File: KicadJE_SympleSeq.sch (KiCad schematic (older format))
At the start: 32 parts, among them J101 CV-Out, J102 Reset + Step, J103 CV-G8_Mod1, J104 CV-G8_Mod2, J105 Clk_Hold, J106 G8-Out, J107 Reset + Step 1-4, J108 Reset + Step 5-8, J109 CV-G8_Base, U101 TL082

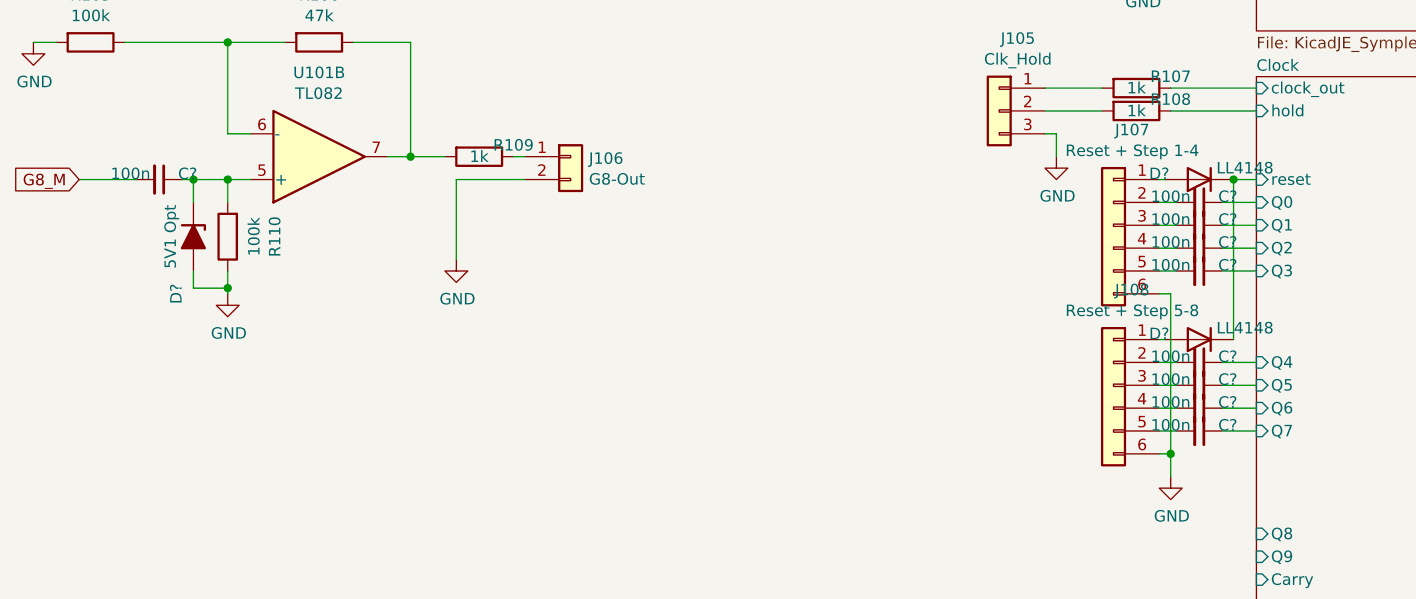
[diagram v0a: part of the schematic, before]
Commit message: ERC Rev B
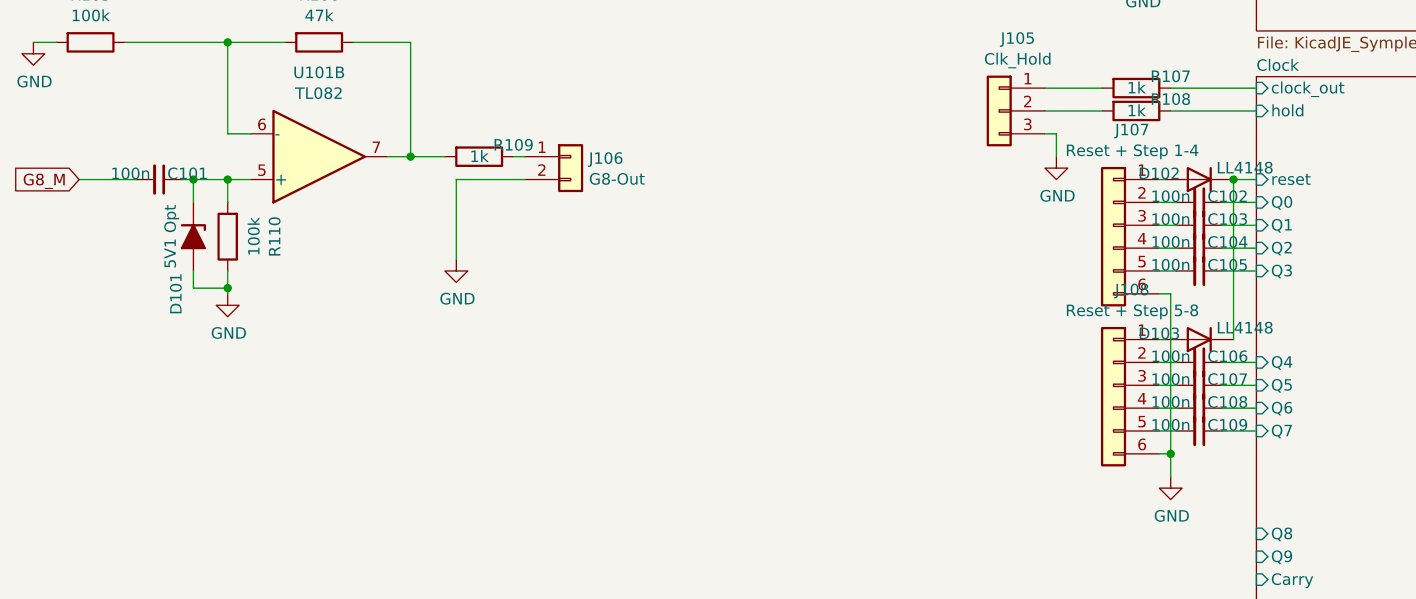
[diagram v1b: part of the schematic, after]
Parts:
- gave numbers to parts that had none: 12
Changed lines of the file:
@@
 	6575 3600 6600 3600
 $Comp
-L Device:C_Small C?
+L Device:C_Small C102
 U 1 1 5EA9D3AA
 P 6750 3700
-F 0 "C?" V 6725 3825 50  0000 C CNN
+F 0 "C102" V 6725 3825 50  0000 C CNN
 F 1 "100n" V 6725 3575 50  0000 C CNN
 F 2 "Capacitor_SMD:C_0805_2012Metric" H 6750 3700 50  0001 C CNN
@@
 	6575 3800 6650 3800
 $Comp
-L Device:C_Small C?
+L Device:C_Small C103
 U 1 1 5EA9ECF0
 P 6750 3800
-F 0 "C?" V 6725 3925 50  0000 C CNN
+F 0 "C103" V 6725 3925 50  0000 C CNN
 F 1 "100n" V 6725 3675 50  0000 C CNN
 F 2 "Capacitor_SMD:C_0805_2012Metric" H 6750 3800 50  0001 C CNN
@@
 	6850 3800 7000 3800
 $Comp
-L Device:C_Small C?
+L Device:C_Small C104
 U 1 1 5EA9F088
 P 6750 3900
-F 0 "C?" V 6725 4025 50  0000 C CNN
+F 0 "C104" V 6725 4025 50  0000 C CNN
 F 1 "100n" V 6725 3775 50  0000 C CNN
 F 2 "Capacitor_SMD:C_0805_2012Metric" H 6750 3900 50  0001 C CNN
@@
 	6850 3900 7000 3900
 $Comp
-L Device:C_Small C?
+L Device:C_Small C105
 U 1 1 5EA9F2B1
 P 6750 4000
-F 0 "C?" V 6725 4125 50  0000 C CNN
+F 0 "C105" V 6725 4125 50  0000 C CNN
 F 1 "100n" V 6725 3875 50  0000 C CNN
 F 2 "Capacitor_SMD:C_0805_2012Metric" H 6750 4000 50  0001 C CNN
@@
 	6850 4000 7000 4000
 $Comp
-L Device:C_Small C?
+L Device:C_Small C106
 U 1 1 5EA9F4B3
 P 6750 4400
-F 0 "C?" V 6725 4525 50  0000 C CNN
+F 0 "C106" V 6725 4525 50  0000 C CNN
 F 1 "100n" V 6725 4275 50  0000 C CNN
 F 2 "Capacitor_SMD:C_0805_2012Metric" H 6750 4400 50  0001 C CNN
@@
 	6850 4400 7000 4400
 $Comp
-L Device:C_Small C?
+L Device:C_Small C107
 U 1 1 5EA9F9A4
 P 6750 4500
-F 0 "C?" V 6725 4625 50  0000 C CNN
+F 0 "C107" V 6725 4625 50  0000 C CNN
 F 1 "100n" V 6725 4375 50  0000 C CNN
 F 2 "Capacitor_SMD:C_0805_2012Metric" H 6750 4500 50  0001 C CNN
@@
 	6850 4500 7000 4500
 $Comp
-L Device:C_Small C?
+L Device:C_Small C108
 U 1 1 5EA9FCDB
 P 6750 4600
-F 0 "C?" V 6725 4725 50  0000 C CNN
+F 0 "C108" V 6725 4725 50  0000 C CNN
 F 1 "100n" V 6725 4475 50  0000 C CNN
 F 2 "Capacitor_SMD:C_0805_2012Metric" H 6750 4600 50  0001 C CNN
@@
 	6850 4600 7000 4600
 $Comp
-L Device:C_Small C?
+L Device:C_Small C109
 U 1 1 5EA9FEC4
 P 6750 4700
-F 0 "C?" V 6725 4825 50  0000 C CNN
+F 0 "C109" V 6725 4825 50  0000 C CNN
 F 1 "100n" V 6725 4575 50  0000 C CNN
 F 2 "Capacitor_SMD:C_0805_2012Metric" H 6750 4700 50  0001 C CNN
@@
 	6850 4700 7000 4700
 $Comp
-L Device:C_Small C?
+L Device:C_Small C101
 U 1 1 5EAA1054
 P 2200 3600
-F 0 "C?" V 2175 3725 50  0000 C CNN
+F 0 "C101" V 2175 3725 50  0000 C CNN
 F 1 "100n" V 2175 3475 50  0000 C CNN
 F 2 "Capacitor_SMD:C_0805_2012Metric" H 2200 3600 50  0001 C CNN
@@
 P 6750 4300
 AR Path="/5C8BFBBC/5EBDB059" Ref="D?"  Part="1"
-AR Path="/5EBDB059" Ref="D?"  Part="1"
-F 0 "D?" H 6925 4275 50  0000 C CNN
+AR Path="/5EBDB059" Ref="D103"  Part="1"
+F 0 "D103" H 6925 4275 50  0000 C CNN
 F 1 "LL4148" H 6550 4250 50  0000 C CNN
 F 2 "Diode_SMD:D_MiniMELF" H 6750 4125 50  0001 C CNN
@@
 P 6750 3600
 AR Path="/5C8BFBBC/5EBDDE8B" Ref="D?"  Part="1"
-AR Path="/5EBDDE8B" Ref="D?"  Part="1"
-F 0 "D?" H 6925 3575 50  0000 C CNN
+AR Path="/5EBDDE8B" Ref="D102"  Part="1"
+F 0 "D102" H 6925 3575 50  0000 C CNN
 F 1 "LL4148" H 6550 3550 50  0000 C CNN
 F 2 "Diode_SMD:D_MiniMELF" H 6750 3425 50  0001 C CNN
@@
 P 2350 3850
 AR Path="/5C8BFBBC/5EBE23F1" Ref="D?"  Part="1"
-AR Path="/5EBE23F1" Ref="D?"  Part="1"
-F 0 "D?" H 2600 3775 50  0000 C CNN
+AR Path="/5EBE23F1" Ref="D101"  Part="1"
+F 0 "D101" H 2600 3775 50  0000 C CNN
 F 1 "5V1 Opt" H 2350 3750 50  0000 C CNN
 F 2 "Diode_SMD:D_MiniMELF" H 2350 3675 50  0001 C CNN

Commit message: AJ Footprints
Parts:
- C101, C102, C103, C104, C105, C106, C107, C108, C109: footprint Capacitor_SMD:C_0805_2012Metric -> AJ:C_0805_2012Metric_Pad1.15x1.40mm_HandSolder
- R101, R102, R103, R104, R105, R106, R107, R108, R109, R110: footprint Resistor_SMD:R_0805_2012Metric_Pad1.15x1.40mm_HandSolder -> AJ:R_0805_2012Metric_Pad1.15x1.40mm_HandSolder
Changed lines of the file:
@@
 F 0 "R106" V 2693 3000 50  0000 C CNN
 F 1 "47k" V 2784 3000 50  0000 C CNN
-F 2 "Resistor_SMD:R_0805_2012Metric_Pad1.15x1.40mm_HandSolder" V 2830 3000 50  0001 C CNN
+F 2 "AJ:R_0805_2012Metric_Pad1.15x1.40mm_HandSolder" V 2830 3000 50  0001 C CNN
 F 3 "~" H 2900 3000 50  0001 C CNN
 	1    2900 3000
@@
 F 0 "R105" V 1693 3000 50  0000 C CNN
 F 1 "100k" V 1784 3000 50  0000 C CNN
-F 2 "Resistor_SMD:R_0805_2012Metric_Pad1.15x1.40mm_HandSolder" V 1830 3000 50  0001 C CNN
+F 2 "AJ:R_0805_2012Metric_Pad1.15x1.40mm_HandSolder" V 1830 3000 50  0001 C CNN
 F 3 "~" H 1900 3000 50  0001 C CNN
 	1    1900 3000
@@
 F 0 "R110" V 2293 3850 50  0000 C CNN
 F 1 "100k" V 2384 3850 50  0000 C CNN
-F 2 "Resistor_SMD:R_0805_2012Metric_Pad1.15x1.40mm_HandSolder" V 2430 3850 50  0001 C CNN
+F 2 "AJ:R_0805_2012Metric_Pad1.15x1.40mm_HandSolder" V 2430 3850 50  0001 C CNN
 F 3 "~" H 2500 3850 50  0001 C CNN
 	1    2500 3850
@@
 F 0 "R107" V 6425 3350 50  0000 C CNN
 F 1 "1k" V 6475 3200 50  0000 C CNN
-F 2 "Resistor_SMD:R_0805_2012Metric_Pad1.15x1.40mm_HandSolder" V 6405 3200 50  0001 C CNN
+F 2 "AJ:R_0805_2012Metric_Pad1.15x1.40mm_HandSolder" V 6405 3200 50  0001 C CNN
 F 3 "~" H 6475 3200 50  0001 C CNN
 	1    6475 3200
@@
 F 0 "R108" V 6425 3450 50  0000 C CNN
 F 1 "1k" V 6475 3300 50  0000 C CNN
-F 2 "Resistor_SMD:R_0805_2012Metric_Pad1.15x1.40mm_HandSolder" V 6405 3300 50  0001 C CNN
+F 2 "AJ:R_0805_2012Metric_Pad1.15x1.40mm_HandSolder" V 6405 3300 50  0001 C CNN
 F 3 "~" H 6475 3300 50  0001 C CNN
 	1    6475 3300
@@
 F 0 "R102" V 2693 1150 50  0000 C CNN
 F 1 "47k" V 2784 1150 50  0000 C CNN
-F 2 "Resistor_SMD:R_0805_2012Metric_Pad1.15x1.40mm_HandSolder" V 2830 1150 50  0001 C CNN
+F 2 "AJ:R_0805_2012Metric_Pad1.15x1.40mm_HandSolder" V 2830 1150 50  0001 C CNN
 F 3 "~" H 2900 1150 50  0001 C CNN
 	1    2900 1150
@@
 F 0 "R104" V 2293 2000 50  0000 C CNN
 F 1 "100k" V 2384 2000 50  0000 C CNN
-F 2 "Resistor_SMD:R_0805_2012Metric_Pad1.15x1.40mm_HandSolder" V 2430 2000 50  0001 C CNN
+F 2 "AJ:R_0805_2012Metric_Pad1.15x1.40mm_HandSolder" V 2430 2000 50  0001 C CNN
 F 3 "~" H 2500 2000 50  0001 C CNN
 	1    2500 2000
@@
 F 0 "R101" V 1693 1150 50  0000 C CNN
 F 1 "100k" V 1784 1150 50  0000 C CNN
-F 2 "Resistor_SMD:R_0805_2012Metric_Pad1.15x1.40mm_HandSolder" V 1830 1150 50  0001 C CNN
+F 2 "AJ:R_0805_2012Metric_Pad1.15x1.40mm_HandSolder" V 1830 1150 50  0001 C CNN
 F 3 "~" H 1900 1150 50  0001 C CNN
 	1    1900 1150
@@
 F 0 "R109" V 3550 3650 50  0000 C CNN
 F 1 "1k" V 3600 3500 50  0000 C CNN
-F 2 "Resistor_SMD:R_0805_2012Metric_Pad1.15x1.40mm_HandSolder" V 3530 3500 50  0001 C CNN
+F 2 "AJ:R_0805_2012Metric_Pad1.15x1.40mm_HandSolder" V 3530 3500 50  0001 C CNN
 F 3 "~" H 3600 3500 50  0001 C CNN
 	1    3600 3500
@@
 F 0 "R103" V 3550 1800 50  0000 C CNN
 F 1 "1k" V 3600 1650 50  0000 C CNN
-F 2 "Resistor_SMD:R_0805_2012Metric_Pad1.15x1.40mm_HandSolder" V 3530 1650 50  0001 C CNN
+F 2 "AJ:R_0805_2012Metric_Pad1.15x1.40mm_HandSolder" V 3530 1650 50  0001 C CNN
 F 3 "~" H 3600 1650 50  0001 C CNN
 	1    3600 1650
@@
 F 0 "C102" V 6725 3825 50  0000 C CNN
 F 1 "100n" V 6725 3575 50  0000 C CNN
-F 2 "Capacitor_SMD:C_0805_2012Metric" H 6750 3700 50  0001 C CNN
+F 2 "AJ:C_0805_2012Metric_Pad1.15x1.40mm_HandSolder" H 6750 3700 50  0001 C CNN
 F 3 "~" H 6750 3700 50  0001 C CNN
 	1    6750 3700
@@
 F 0 "C103" V 6725 3925 50  0000 C CNN
 F 1 "100n" V 6725 3675 50  0000 C CNN
-F 2 "Capacitor_SMD:C_0805_2012Metric" H 6750 3800 50  0001 C CNN
+F 2 "AJ:C_0805_2012Metric_Pad1.15x1.40mm_HandSolder" H 6750 3800 50  0001 C CNN
 F 3 "~" H 6750 3800 50  0001 C CNN
 	1    6750 3800
@@
 F 0 "C104" V 6725 4025 50  0000 C CNN
 F 1 "100n" V 6725 3775 50  0000 C CNN
-F 2 "Capacitor_SMD:C_0805_2012Metric" H 6750 3900 50  0001 C CNN
+F 2 "AJ:C_0805_2012Metric_Pad1.15x1.40mm_HandSolder" H 6750 3900 50  0001 C CNN
 F 3 "~" H 6750 3900 50  0001 C CNN
 	1    6750 3900
@@
 F 0 "C105" V 6725 4125 50  0000 C CNN
 F 1 "100n" V 6725 3875 50  0000 C CNN
-F 2 "Capacitor_SMD:C_0805_2012Metric" H 6750 4000 50  0001 C CNN
+F 2 "AJ:C_0805_2012Metric_Pad1.15x1.40mm_HandSolder" H 6750 4000 50  0001 C CNN
 F 3 "~" H 6750 4000 50  0001 C CNN
 	1    6750 4000
@@
 F 0 "C106" V 6725 4525 50  0000 C CNN
 F 1 "100n" V 6725 4275 50  0000 C CNN
-F 2 "Capacitor_SMD:C_0805_2012Metric" H 6750 4400 50  0001 C CNN
+F 2 "AJ:C_0805_2012Metric_Pad1.15x1.40mm_HandSolder" H 6750 4400 50  0001 C CNN
 F 3 "~" H 6750 4400 50  0001 C CNN
 	1    6750 4400
@@
 F 0 "C107" V 6725 4625 50  0000 C CNN
 F 1 "100n" V 6725 4375 50  0000 C CNN
-F 2 "Capacitor_SMD:C_0805_2012Metric" H 6750 4500 50  0001 C CNN
+F 2 "AJ:C_0805_2012Metric_Pad1.15x1.40mm_HandSolder" H 6750 4500 50  0001 C CNN
 F 3 "~" H 6750 4500 50  0001 C CNN
 	1    6750 4500
@@
 F 0 "C108" V 6725 4725 50  0000 C CNN
 F 1 "100n" V 6725 4475 50  0000 C CNN
-F 2 "Capacitor_SMD:C_0805_2012Metric" H 6750 4600 50  0001 C CNN
+F 2 "AJ:C_0805_2012Metric_Pad1.15x1.40mm_HandSolder" H 6750 4600 50  0001 C CNN
 F 3 "~" H 6750 4600 50  0001 C CNN
 	1    6750 4600
@@
 F 0 "C109" V 6725 4825 50  0000 C CNN
 F 1 "100n" V 6725 4575 50  0000 C CNN
-F 2 "Capacitor_SMD:C_0805_2012Metric" H 6750 4700 50  0001 C CNN
+F 2 "AJ:C_0805_2012Metric_Pad1.15x1.40mm_HandSolder" H 6750 4700 50  0001 C CNN
 F 3 "~" H 6750 4700 50  0001 C CNN
 	1    6750 4700
@@
 F 0 "C101" V 2175 3725 50  0000 C CNN
 F 1 "100n" V 2175 3475 50  0000 C CNN
-F 2 "Capacitor_SMD:C_0805_2012Metric" H 2200 3600 50  0001 C CNN
+F 2 "AJ:C_0805_2012Metric_Pad1.15x1.40mm_HandSolder" H 2200 3600 50  0001 C CNN
 F 3 "~" H 2200 3600 50  0001 C CNN
 	1    2200 3600

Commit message: AJ footprints updated
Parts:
- C101, C102, C103, C104, C105, C106, C107, C108, C109: footprint AJ:C_0805_2012Metric_Pad1.15x1.40mm_HandSolder -> AJ:C_0805_AJ
- R101, R102, R103, R104, R105, R106, R107, R108, R109, R110: footprint AJ:R_0805_2012Metric_Pad1.15x1.40mm_HandSolder -> AJ:R_0805_AJ
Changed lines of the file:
@@
 F 0 "R106" V 2693 3000 50  0000 C CNN
 F 1 "47k" V 2784 3000 50  0000 C CNN
-F 2 "AJ:R_0805_2012Metric_Pad1.15x1.40mm_HandSolder" V 2830 3000 50  0001 C CNN
+F 2 "AJ:R_0805_AJ" V 2830 3000 50  0001 C CNN
 F 3 "~" H 2900 3000 50  0001 C CNN
 	1    2900 3000
@@
 F 0 "R105" V 1693 3000 50  0000 C CNN
 F 1 "100k" V 1784 3000 50  0000 C CNN
-F 2 "AJ:R_0805_2012Metric_Pad1.15x1.40mm_HandSolder" V 1830 3000 50  0001 C CNN
+F 2 "AJ:R_0805_AJ" V 1830 3000 50  0001 C CNN
 F 3 "~" H 1900 3000 50  0001 C CNN
 	1    1900 3000
@@
 F 0 "R110" V 2293 3850 50  0000 C CNN
 F 1 "100k" V 2384 3850 50  0000 C CNN
-F 2 "AJ:R_0805_2012Metric_Pad1.15x1.40mm_HandSolder" V 2430 3850 50  0001 C CNN
+F 2 "AJ:R_0805_AJ" V 2430 3850 50  0001 C CNN
 F 3 "~" H 2500 3850 50  0001 C CNN
 	1    2500 3850
@@
 F 0 "R107" V 6425 3350 50  0000 C CNN
 F 1 "1k" V 6475 3200 50  0000 C CNN
-F 2 "AJ:R_0805_2012Metric_Pad1.15x1.40mm_HandSolder" V 6405 3200 50  0001 C CNN
+F 2 "AJ:R_0805_AJ" V 6405 3200 50  0001 C CNN
 F 3 "~" H 6475 3200 50  0001 C CNN
 	1    6475 3200
@@
 F 0 "R108" V 6425 3450 50  0000 C CNN
 F 1 "1k" V 6475 3300 50  0000 C CNN
-F 2 "AJ:R_0805_2012Metric_Pad1.15x1.40mm_HandSolder" V 6405 3300 50  0001 C CNN
+F 2 "AJ:R_0805_AJ" V 6405 3300 50  0001 C CNN
 F 3 "~" H 6475 3300 50  0001 C CNN
 	1    6475 3300
@@
 F 0 "R102" V 2693 1150 50  0000 C CNN
 F 1 "47k" V 2784 1150 50  0000 C CNN
-F 2 "AJ:R_0805_2012Metric_Pad1.15x1.40mm_HandSolder" V 2830 1150 50  0001 C CNN
+F 2 "AJ:R_0805_AJ" V 2830 1150 50  0001 C CNN
 F 3 "~" H 2900 1150 50  0001 C CNN
 	1    2900 1150
@@
 F 0 "R104" V 2293 2000 50  0000 C CNN
 F 1 "100k" V 2384 2000 50  0000 C CNN
-F 2 "AJ:R_0805_2012Metric_Pad1.15x1.40mm_HandSolder" V 2430 2000 50  0001 C CNN
+F 2 "AJ:R_0805_AJ" V 2430 2000 50  0001 C CNN
 F 3 "~" H 2500 2000 50  0001 C CNN
 	1    2500 2000
@@
 F 0 "R101" V 1693 1150 50  0000 C CNN
 F 1 "100k" V 1784 1150 50  0000 C CNN
-F 2 "AJ:R_0805_2012Metric_Pad1.15x1.40mm_HandSolder" V 1830 1150 50  0001 C CNN
+F 2 "AJ:R_0805_AJ" V 1830 1150 50  0001 C CNN
 F 3 "~" H 1900 1150 50  0001 C CNN
 	1    1900 1150
@@
 F 0 "R109" V 3550 3650 50  0000 C CNN
 F 1 "1k" V 3600 3500 50  0000 C CNN
-F 2 "AJ:R_0805_2012Metric_Pad1.15x1.40mm_HandSolder" V 3530 3500 50  0001 C CNN
+F 2 "AJ:R_0805_AJ" V 3530 3500 50  0001 C CNN
 F 3 "~" H 3600 3500 50  0001 C CNN
 	1    3600 3500
@@
 F 0 "R103" V 3550 1800 50  0000 C CNN
 F 1 "1k" V 3600 1650 50  0000 C CNN
-F 2 "AJ:R_0805_2012Metric_Pad1.15x1.40mm_HandSolder" V 3530 1650 50  0001 C CNN
+F 2 "AJ:R_0805_AJ" V 3530 1650 50  0001 C CNN
 F 3 "~" H 3600 1650 50  0001 C CNN
 	1    3600 1650
@@
 F 0 "C102" V 6725 3825 50  0000 C CNN
 F 1 "100n" V 6725 3575 50  0000 C CNN
-F 2 "AJ:C_0805_2012Metric_Pad1.15x1.40mm_HandSolder" H 6750 3700 50  0001 C CNN
+F 2 "AJ:C_0805_AJ" H 6750 3700 50  0001 C CNN
 F 3 "~" H 6750 3700 50  0001 C CNN
 	1    6750 3700
@@
 F 0 "C103" V 6725 3925 50  0000 C CNN
 F 1 "100n" V 6725 3675 50  0000 C CNN
-F 2 "AJ:C_0805_2012Metric_Pad1.15x1.40mm_HandSolder" H 6750 3800 50  0001 C CNN
+F 2 "AJ:C_0805_AJ" H 6750 3800 50  0001 C CNN
 F 3 "~" H 6750 3800 50  0001 C CNN
 	1    6750 3800
@@
 F 0 "C104" V 6725 4025 50  0000 C CNN
 F 1 "100n" V 6725 3775 50  0000 C CNN
-F 2 "AJ:C_0805_2012Metric_Pad1.15x1.40mm_HandSolder" H 6750 3900 50  0001 C CNN
+F 2 "AJ:C_0805_AJ" H 6750 3900 50  0001 C CNN
 F 3 "~" H 6750 3900 50  0001 C CNN
 	1    6750 3900
@@
 F 0 "C105" V 6725 4125 50  0000 C CNN
 F 1 "100n" V 6725 3875 50  0000 C CNN
-F 2 "AJ:C_0805_2012Metric_Pad1.15x1.40mm_HandSolder" H 6750 4000 50  0001 C CNN
+F 2 "AJ:C_0805_AJ" H 6750 4000 50  0001 C CNN
 F 3 "~" H 6750 4000 50  0001 C CNN
 	1    6750 4000
@@
 F 0 "C106" V 6725 4525 50  0000 C CNN
 F 1 "100n" V 6725 4275 50  0000 C CNN
-F 2 "AJ:C_0805_2012Metric_Pad1.15x1.40mm_HandSolder" H 6750 4400 50  0001 C CNN
+F 2 "AJ:C_0805_AJ" H 6750 4400 50  0001 C CNN
 F 3 "~" H 6750 4400 50  0001 C CNN
 	1    6750 4400
@@
 F 0 "C107" V 6725 4625 50  0000 C CNN
 F 1 "100n" V 6725 4375 50  0000 C CNN
-F 2 "AJ:C_0805_2012Metric_Pad1.15x1.40mm_HandSolder" H 6750 4500 50  0001 C CNN
+F 2 "AJ:C_0805_AJ" H 6750 4500 50  0001 C CNN
 F 3 "~" H 6750 4500 50  0001 C CNN
 	1    6750 4500
@@
 F 0 "C108" V 6725 4725 50  0000 C CNN
 F 1 "100n" V 6725 4475 50  0000 C CNN
-F 2 "AJ:C_0805_2012Metric_Pad1.15x1.40mm_HandSolder" H 6750 4600 50  0001 C CNN
+F 2 "AJ:C_0805_AJ" H 6750 4600 50  0001 C CNN
 F 3 "~" H 6750 4600 50  0001 C CNN
 	1    6750 4600
@@
 F 0 "C109" V 6725 4825 50  0000 C CNN
 F 1 "100n" V 6725 4575 50  0000 C CNN
-F 2 "AJ:C_0805_2012Metric_Pad1.15x1.40mm_HandSolder" H 6750 4700 50  0001 C CNN
+F 2 "AJ:C_0805_AJ" H 6750 4700 50  0001 C CNN
 F 3 "~" H 6750 4700 50  0001 C CNN
 	1    6750 4700
@@
 F 0 "C101" V 2175 3725 50  0000 C CNN
 F 1 "100n" V 2175 3475 50  0000 C CNN
-F 2 "AJ:C_0805_2012Metric_Pad1.15x1.40mm_HandSolder" H 2200 3600 50  0001 C CNN
+F 2 "AJ:C_0805_AJ" H 2200 3600 50  0001 C CNN
 F 3 "~" H 2200 3600 50  0001 C CNN
 	1    2200 3600
